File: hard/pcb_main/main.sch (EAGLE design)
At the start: 184 parts

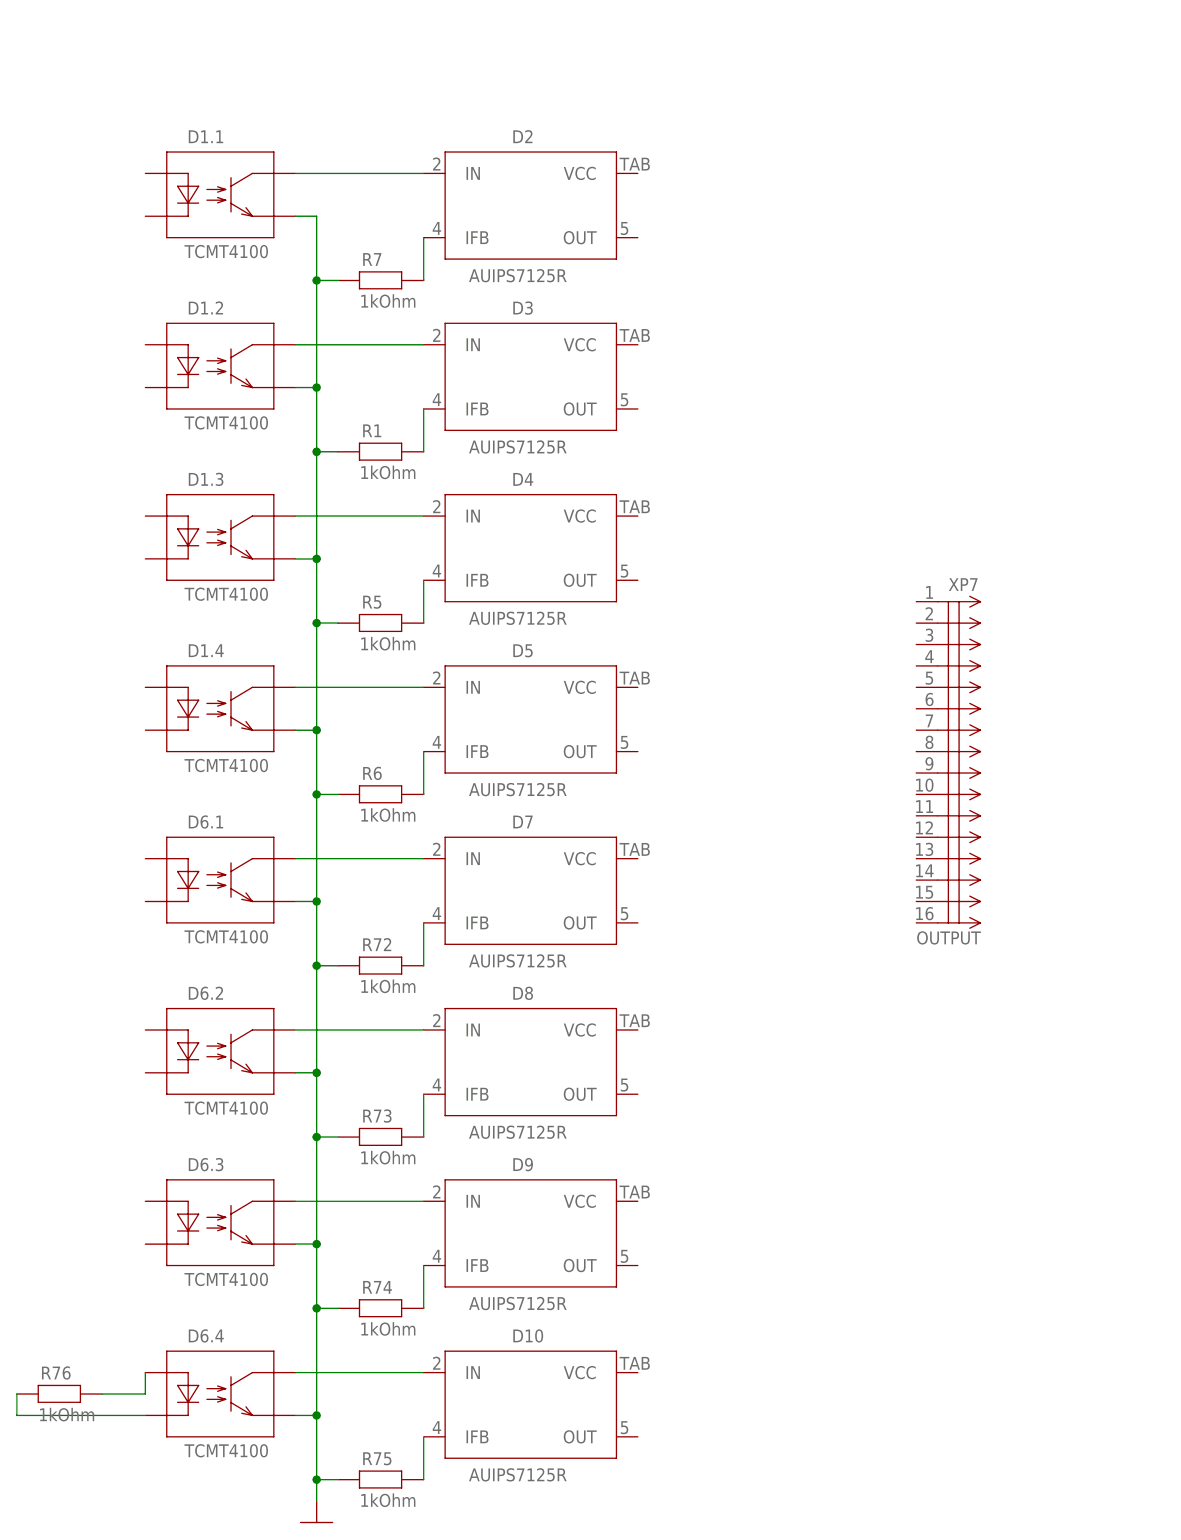
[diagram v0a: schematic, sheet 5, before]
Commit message: output schematic improvemetns
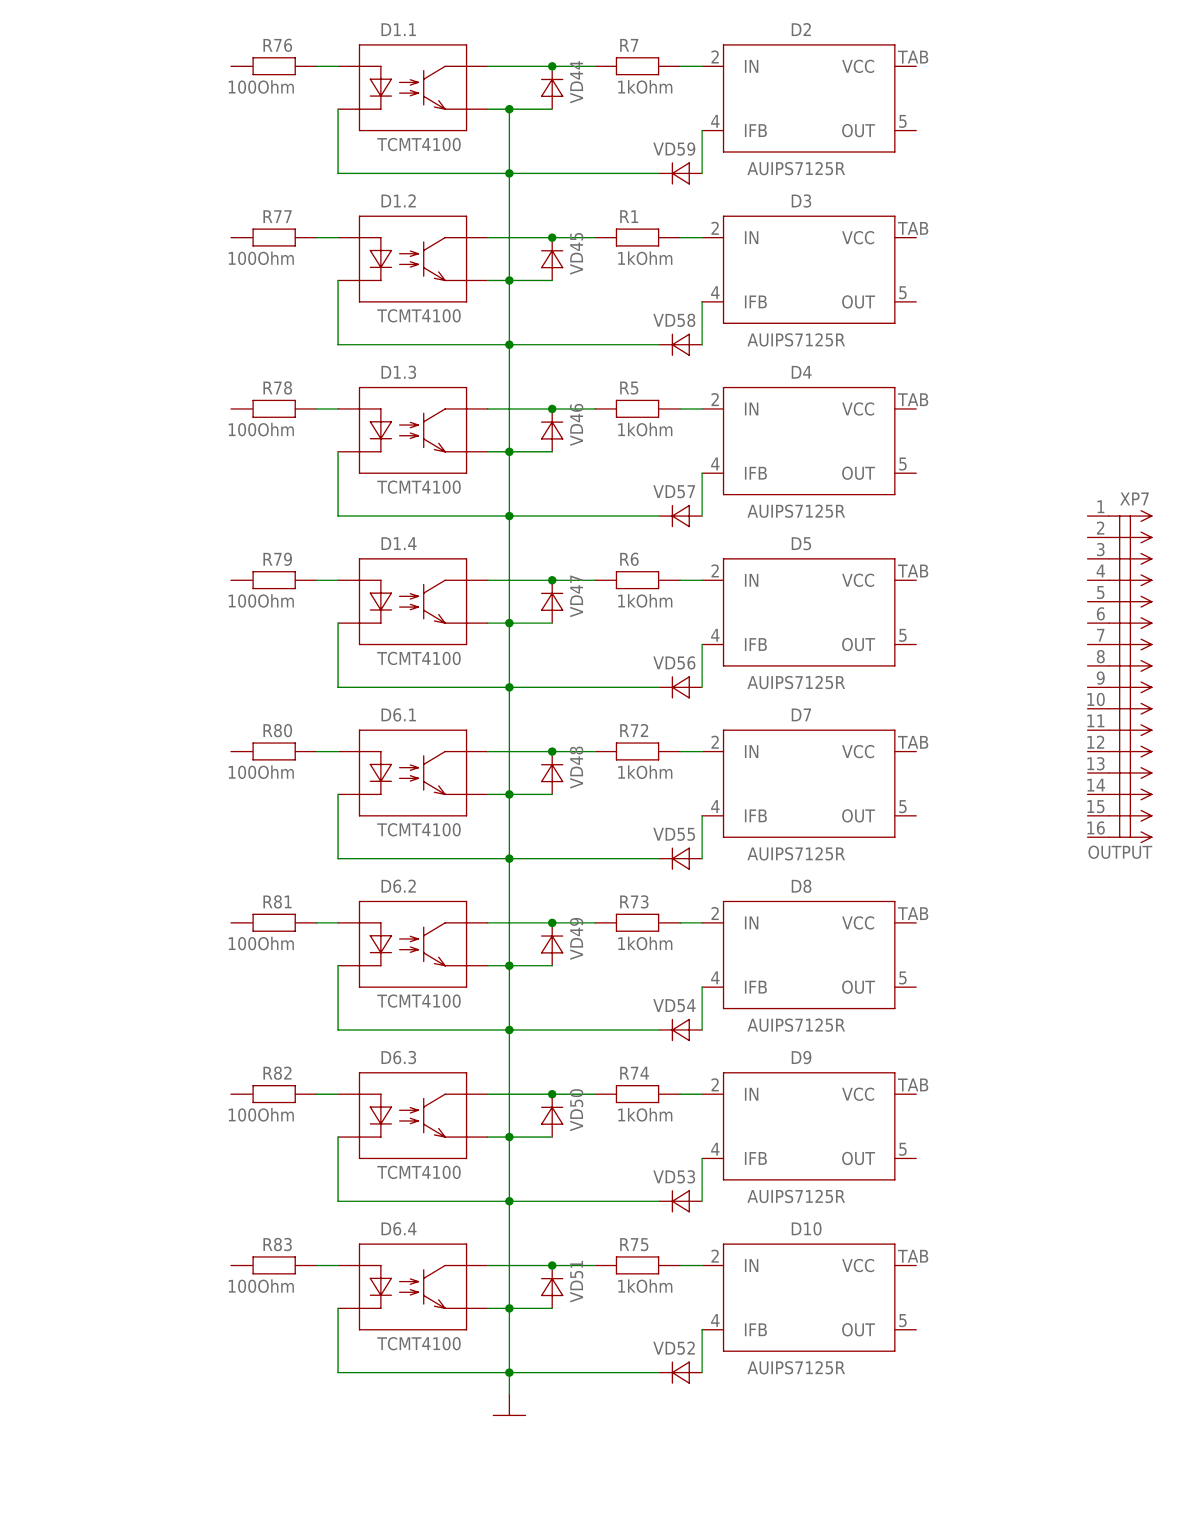
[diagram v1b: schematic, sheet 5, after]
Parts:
- added R77, R78, R79, R80, R81, R82, R83: 100Ohm, rcl:R-EU_R0603
- added VD44, VD45, VD46, VD47, VD48, VD49, VD50, VD51, VD52, VD53, VD54, VD55, VD56, VD57, VD58, VD59: (no value), diode:DIODE-STANDARD-SOD323
- R76: value 1kOhm -> 100Ohm; device rcl:R-EU_R0805 -> rcl:R-EU_R0603; PARTNO ERJ6GEYJ102V -> ERJ3GEYJ101V
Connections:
- new net N$55: D6.2.DA, R81.1
- new net N$56: D6.1.DA, R80.1
- new net N$57: D1.4.DA, R79.1
- new net N$58: D1.3.DA, R78.1
- new net N$59: D1.2.DA, R77.1
- new net N$60: D1.1.DA, R76.1
- new net N$62: D2.IFB, VD59.A
- new net N$63: D3.IFB, VD58.A
- new net N$64: D4.IFB, VD57.A
- new net N$65: D5.IFB, VD56.A
- new net N$66: D7.IFB, VD55.A
- new net N$67: D8.IFB, VD54.A
- new net N$68: D9.IFB, VD53.A
- new net N$69: D10.IFB, VD52.A
- net GND: now also D1.1.DC, D1.2.DC, D1.3.DC, D1.4.DC, D6.1.DC, D6.2.DC, D6.3.DC, D6.4.DC, VD44.A, VD45.A, VD46.A, VD47.A, VD48.A, VD49.A, VD50.A, VD51.A, VD52.C, VD53.C, VD54.C, VD55.C, VD56.C, VD57.C, VD58.C, VD59.C; no longer R1.1, R5.1, R6.1, R7.1, R72.1, R73.1, R74.1, R75.1
- net N$1: now also D10.IN, R75.2; no longer D1.1.TC, D2.IN
- net N$10: now also D2.IN; no longer D2.IFB
- net N$11: now also R83.1; no longer R76.2
- net N$3: now also D9.IN, R74.2; no longer D1.2.TC, D3.IN
- net N$4: now also D8.IN, R73.2; no longer D1.3.TC, D4.IN
- net N$46: now also D1.1.TC, R7.1, VD44.C; no longer D6.1.TC, D7.IN
- net N$47: now also D1.2.TC, R1.1, VD45.C; no longer D6.2.TC, D8.IN
- net N$48: now also D1.3.TC, R5.1, VD46.C; no longer D6.3.TC, D9.IN
- net N$49: now also D1.4.TC, R6.1, VD47.C; no longer D10.IN, D6.4.TC
- net N$5: now also D7.IN, R72.2; no longer D1.4.TC, D5.IN
- net N$50: now also D6.1.TC, R72.1, VD48.C; no longer D10.IFB, R75.2
- net N$51: now also D6.2.TC, R73.1, VD49.C; no longer D9.IFB, R74.2
- net N$52: now also D6.3.TC, R74.1, VD50.C; no longer D8.IFB, R73.2
- net N$53: now also D6.4.TC, R75.1, VD51.C; no longer D7.IFB, R72.2
- net N$54: now also D6.3.DA, R82.1; no longer D6.4.DC, R76.1
- net N$6: now also D5.IN; no longer D5.IFB
- net N$8: now also D4.IN; no longer D4.IFB
- net N$9: now also D3.IN; no longer D3.IFB
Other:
- moved on the sheet: D1.1, D1.2, D1.3, D1.4, D10, D2, D3, D4, D5, D6.1, D6.2, D6.3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
